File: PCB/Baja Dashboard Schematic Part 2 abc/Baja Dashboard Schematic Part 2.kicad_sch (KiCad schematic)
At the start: 53 parts, among them J1 Conn_01x04_Pin, J2 Conn_01x04_Pin, Q2 MMBT2222_, SW1 SW_Push, SW2 SW_Push, U1 TLC5917, U2 TLC5917, U3 TLC5917, U9 TLC555xPS

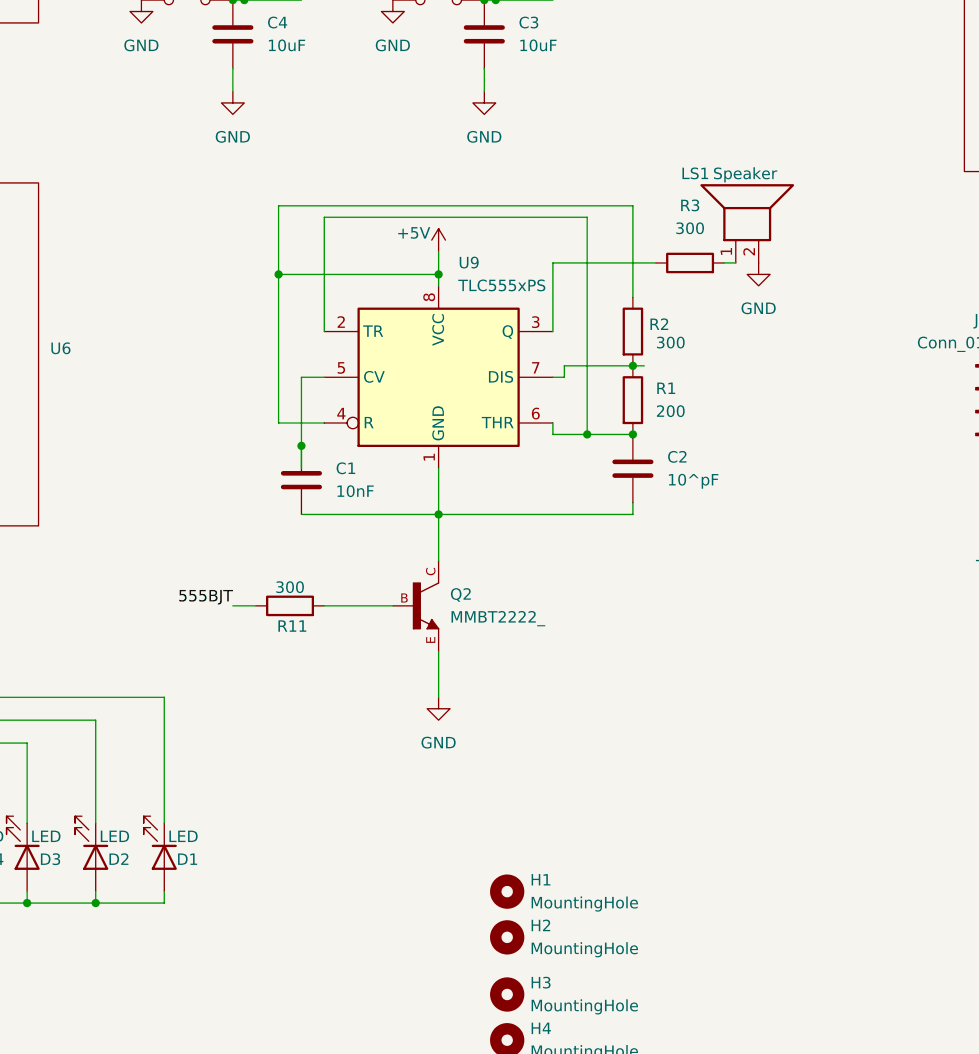
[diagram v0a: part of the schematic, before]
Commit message: Add files via upload
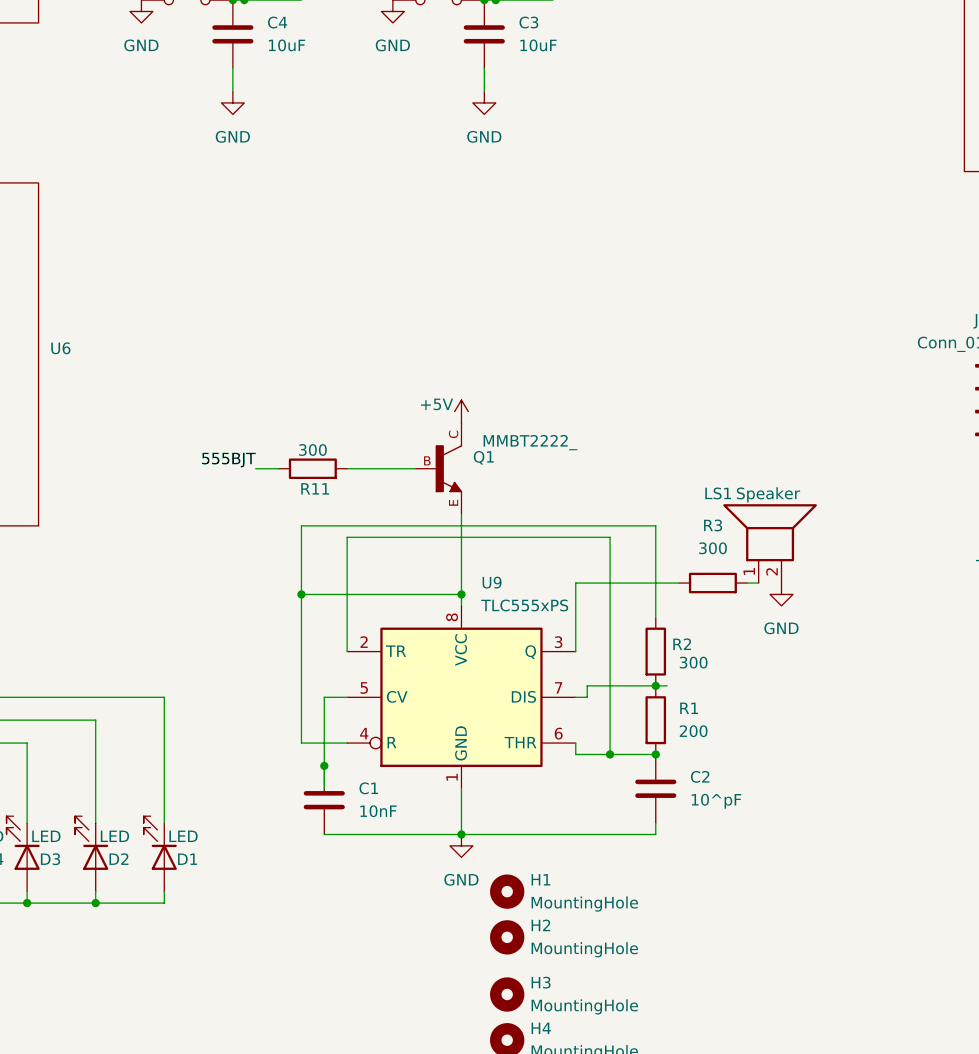
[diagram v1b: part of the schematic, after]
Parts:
- removed Q2: MMBT2222_, bajaRedoSaves:MMBT2222, symbol MMBT2222_:MMBT2222_
- added Q1: MMBT2222_, bajaRedoSaves:MMBT2222, symbol MMBT2222_:MMBT2222_
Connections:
- net +5V: now also Q1.C; no longer R2.1, U9.4 (R), U9.8 (VCC)
- net GND: now also C1.2, C2.2, U9.1 (GND)
- net at R11.2: now also Q1.B
- new net: Q1.E, R2.1, U9.4 (R), U9.8 (VCC)
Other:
- moved on the sheet: C1, C2, R1, R2, R3, U9
